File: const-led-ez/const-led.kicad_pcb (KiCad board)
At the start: 2 copper layers, 25.4 x 25.4 mm, 60 parts, among them CON1 AVR-ISP-6, J1 Micro_USB_B, J2 Conn_01x02, SW1 SW_SPST, SW2 SW_SPST, U1 MCP73831, U2 LM3410, U3 ATTINY85-20SU

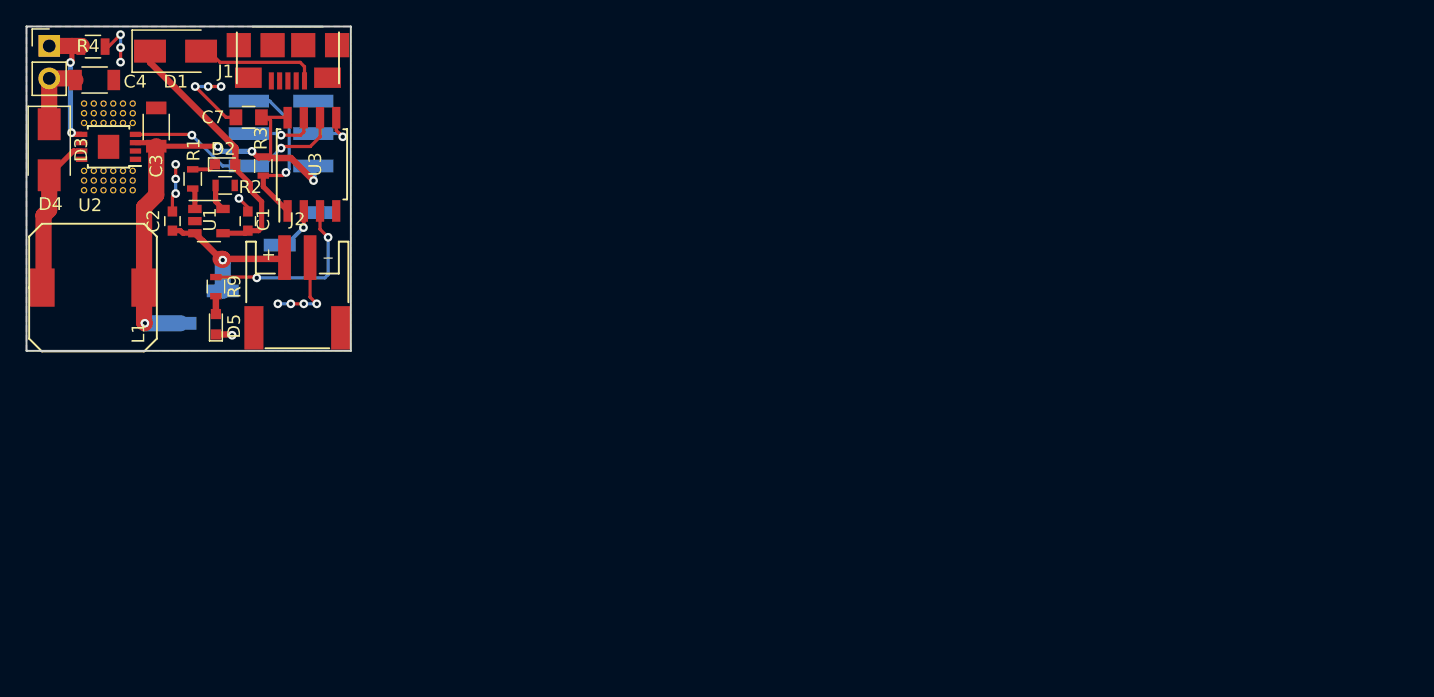
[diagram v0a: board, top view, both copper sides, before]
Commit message: Rev2
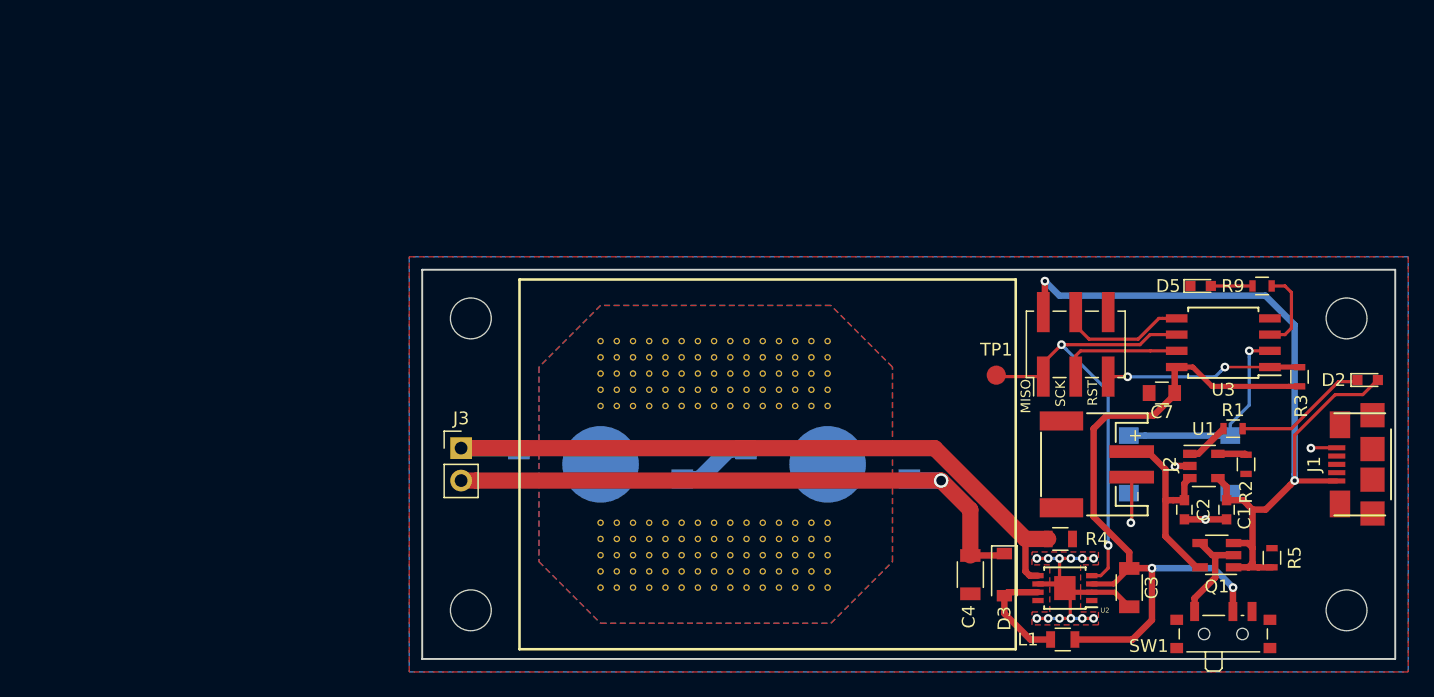
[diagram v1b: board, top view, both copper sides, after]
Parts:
- removed D1: D_Schottky, Diodes_SMD:D_SMA
- removed REF** (x36): VIA-12mil, personal_f:VIA-12mil
- added D6: LED, personal_f:ChanzonLED, B.Cu at (148.6, 111.8)
- added G***: LOGO, personal_f:Guang, B.Cu at (182.3, 111.8)
- added J3: Conn_01x02, Pin_Headers:Pin_Header_Straight_1x02_Pitch2.54mm, F.Cu at (137.7, 110.5)
- added J4: Conn_01x01, Mounting_Holes:MountingHole_3.2mm_M3, F.Cu at (138.4, 123.2)
- added J5: Conn_01x01, Mounting_Holes:MountingHole_3.2mm_M3, F.Cu at (207.0, 123.2)
- added J6: Conn_01x01, Mounting_Holes:MountingHole_3.2mm_M3, F.Cu at (138.4, 100.3)
- added J7: Conn_01x01, Mounting_Holes:MountingHole_3.2mm_M3, F.Cu at (207.0, 100.3)
- added J8: Conn_01x01, personal_f:VIA-12mil, F.Cu at (166.4, 121.4)
- added J8: Conn_01x01, personal_f:VIA-12mil, F.Cu at (154.9, 121.4)
- added J8: Conn_01x01, personal_f:VIA-12mil, F.Cu at (153.7, 121.4)
- added J8: Conn_01x01, personal_f:VIA-12mil, F.Cu at (152.4, 121.4)
- added J8: Conn_01x01, personal_f:VIA-12mil, F.Cu at (151.1, 121.4)
- added J8: Conn_01x01, personal_f:VIA-12mil, F.Cu at (149.9, 121.4)
- added J8: Conn_01x01, personal_f:VIA-12mil, F.Cu at (148.6, 121.4)
- added J8: Conn_01x01, personal_f:VIA-12mil, F.Cu at (166.4, 120.1)
- added J8: Conn_01x01, personal_f:VIA-12mil, F.Cu at (165.1, 120.1)
- added J8: Conn_01x01, personal_f:VIA-12mil, F.Cu at (163.8, 120.1)
- added J8: Conn_01x01, personal_f:VIA-12mil, F.Cu at (162.6, 120.1)
- added J8: Conn_01x01, personal_f:VIA-12mil, F.Cu at (165.1, 121.4)
- added J8: Conn_01x01, personal_f:VIA-12mil, F.Cu at (161.3, 120.1)
- added J8: Conn_01x01, personal_f:VIA-12mil, F.Cu at (160.0, 120.1)
- added J8: Conn_01x01, personal_f:VIA-12mil, F.Cu at (158.8, 120.1)
- added J8: Conn_01x01, personal_f:VIA-12mil, F.Cu at (157.5, 120.1)
- added J8: Conn_01x01, personal_f:VIA-12mil, F.Cu at (156.2, 120.1)
- added J8: Conn_01x01, personal_f:VIA-12mil, F.Cu at (154.9, 120.1)
- added J8: Conn_01x01, personal_f:VIA-12mil, F.Cu at (153.7, 120.1)
- added J8: Conn_01x01, personal_f:VIA-12mil, F.Cu at (152.4, 120.1)
- added J8: Conn_01x01, personal_f:VIA-12mil, F.Cu at (151.1, 120.1)
- added J8: Conn_01x01, personal_f:VIA-12mil, F.Cu at (149.9, 120.1)
- added J8: Conn_01x01, personal_f:VIA-12mil, F.Cu at (163.8, 121.4)
- added J8: Conn_01x01, personal_f:VIA-12mil, F.Cu at (148.6, 120.1)
- added J8: Conn_01x01, personal_f:VIA-12mil, F.Cu at (166.4, 118.9)
- added J8: Conn_01x01, personal_f:VIA-12mil, F.Cu at (165.1, 118.9)
- added J8: Conn_01x01, personal_f:VIA-12mil, F.Cu at (163.8, 118.9)
- added J8: Conn_01x01, personal_f:VIA-12mil, F.Cu at (162.6, 118.9)
- added J8: Conn_01x01, personal_f:VIA-12mil, F.Cu at (161.3, 118.9)
- added J8: Conn_01x01, personal_f:VIA-12mil, F.Cu at (160.0, 118.9)
- added J8: Conn_01x01, personal_f:VIA-12mil, F.Cu at (158.8, 118.9)
- added J8: Conn_01x01, personal_f:VIA-12mil, F.Cu at (157.5, 118.9)
- added J8: Conn_01x01, personal_f:VIA-12mil, F.Cu at (156.2, 118.9)
- added J8: Conn_01x01, personal_f:VIA-12mil, F.Cu at (162.6, 121.4)
- added J8: Conn_01x01, personal_f:VIA-12mil, F.Cu at (154.9, 118.9)
- added J8: Conn_01x01, personal_f:VIA-12mil, F.Cu at (153.7, 118.9)
- added J8: Conn_01x01, personal_f:VIA-12mil, F.Cu at (152.4, 118.9)
- added J8: Conn_01x01, personal_f:VIA-12mil, F.Cu at (151.1, 118.9)
- added J8: Conn_01x01, personal_f:VIA-12mil, F.Cu at (149.9, 118.9)
- added J8: Conn_01x01, personal_f:VIA-12mil, F.Cu at (148.6, 118.9)
- added J8: Conn_01x01, personal_f:VIA-12mil, F.Cu at (166.4, 117.6)
- added J8: Conn_01x01, personal_f:VIA-12mil, F.Cu at (165.1, 117.6)
- added J8: Conn_01x01, personal_f:VIA-12mil, F.Cu at (163.8, 117.6)
- added J8: Conn_01x01, personal_f:VIA-12mil, F.Cu at (162.6, 117.6)
- added J8: Conn_01x01, personal_f:VIA-12mil, F.Cu at (161.3, 121.4)
- added J8: Conn_01x01, personal_f:VIA-12mil, F.Cu at (161.3, 117.6)
- added J8: Conn_01x01, personal_f:VIA-12mil, F.Cu at (160.0, 117.6)
- added J8: Conn_01x01, personal_f:VIA-12mil, F.Cu at (158.8, 117.6)
- added J8: Conn_01x01, personal_f:VIA-12mil, F.Cu at (157.5, 117.6)
- added J8: Conn_01x01, personal_f:VIA-12mil, F.Cu at (156.2, 117.6)
- added J8: Conn_01x01, personal_f:VIA-12mil, F.Cu at (154.9, 117.6)
- added J8: Conn_01x01, personal_f:VIA-12mil, F.Cu at (153.7, 117.6)
- added J8: Conn_01x01, personal_f:VIA-12mil, F.Cu at (152.4, 117.6)
- added J8: Conn_01x01, personal_f:VIA-12mil, F.Cu at (151.1, 117.6)
- added J8: Conn_01x01, personal_f:VIA-12mil, F.Cu at (149.9, 117.6)
- added J8: Conn_01x01, personal_f:VIA-12mil, F.Cu at (160.0, 121.4)
- added J8: Conn_01x01, personal_f:VIA-12mil, F.Cu at (148.6, 117.6)
- added J8: Conn_01x01, personal_f:VIA-12mil, F.Cu at (166.4, 116.3)
- added J8: Conn_01x01, personal_f:VIA-12mil, F.Cu at (165.1, 116.3)
- added J8: Conn_01x01, personal_f:VIA-12mil, F.Cu at (163.8, 116.3)
- added J8: Conn_01x01, personal_f:VIA-12mil, F.Cu at (162.6, 116.3)
- added J8: Conn_01x01, personal_f:VIA-12mil, F.Cu at (161.3, 116.3)
- added J8: Conn_01x01, personal_f:VIA-12mil, F.Cu at (160.0, 116.3)
- added J8: Conn_01x01, personal_f:VIA-12mil, F.Cu at (158.8, 116.3)
- added J8: Conn_01x01, personal_f:VIA-12mil, F.Cu at (157.5, 116.3)
- added J8: Conn_01x01, personal_f:VIA-12mil, F.Cu at (156.2, 116.3)
- added J8: Conn_01x01, personal_f:VIA-12mil, F.Cu at (158.8, 121.4)
- added J8: Conn_01x01, personal_f:VIA-12mil, F.Cu at (154.9, 116.3)
- added J8: Conn_01x01, personal_f:VIA-12mil, F.Cu at (153.7, 116.3)
- added J8: Conn_01x01, personal_f:VIA-12mil, F.Cu at (152.4, 116.3)
- added J8: Conn_01x01, personal_f:VIA-12mil, F.Cu at (151.1, 116.3)
- added J8: Conn_01x01, personal_f:VIA-12mil, F.Cu at (149.9, 116.3)
- added J8: Conn_01x01, personal_f:VIA-12mil, F.Cu at (148.6, 116.3)
- added J8: Conn_01x01, personal_f:VIA-12mil, F.Cu at (157.5, 121.4)
- added J8: Conn_01x01, personal_f:VIA-12mil, F.Cu at (156.2, 121.4)
- added J9: Conn_01x01, personal_f:VIA-12mil, F.Cu at (166.4, 102.1)
- added J9: Conn_01x01, personal_f:VIA-12mil, F.Cu at (154.9, 102.1)
- added J9: Conn_01x01, personal_f:VIA-12mil, F.Cu at (153.7, 102.1)
- added J9: Conn_01x01, personal_f:VIA-12mil, F.Cu at (152.4, 102.1)
- added J9: Conn_01x01, personal_f:VIA-12mil, F.Cu at (151.1, 102.1)
- added J9: Conn_01x01, personal_f:VIA-12mil, F.Cu at (149.9, 102.1)
- added J9: Conn_01x01, personal_f:VIA-12mil, F.Cu at (148.6, 102.1)
- added J9: Conn_01x01, personal_f:VIA-12mil, F.Cu at (166.4, 103.4)
- added J9: Conn_01x01, personal_f:VIA-12mil, F.Cu at (165.1, 103.4)
- added J9: Conn_01x01, personal_f:VIA-12mil, F.Cu at (163.8, 103.4)
- added J9: Conn_01x01, personal_f:VIA-12mil, F.Cu at (162.6, 103.4)
- added J9: Conn_01x01, personal_f:VIA-12mil, F.Cu at (165.1, 102.1)
- added J9: Conn_01x01, personal_f:VIA-12mil, F.Cu at (161.3, 103.4)
- added J9: Conn_01x01, personal_f:VIA-12mil, F.Cu at (160.0, 103.4)
- added J9: Conn_01x01, personal_f:VIA-12mil, F.Cu at (158.8, 103.4)
- added J9: Conn_01x01, personal_f:VIA-12mil, F.Cu at (157.5, 103.4)
- added J9: Conn_01x01, personal_f:VIA-12mil, F.Cu at (156.2, 103.4)
- added J9: Conn_01x01, personal_f:VIA-12mil, F.Cu at (154.9, 103.4)
- added J9: Conn_01x01, personal_f:VIA-12mil, F.Cu at (153.7, 103.4)
- added J9: Conn_01x01, personal_f:VIA-12mil, F.Cu at (152.4, 103.4)
- added J9: Conn_01x01, personal_f:VIA-12mil, F.Cu at (151.1, 103.4)
- added J9: Conn_01x01, personal_f:VIA-12mil, F.Cu at (149.9, 103.4)
- added J9: Conn_01x01, personal_f:VIA-12mil, F.Cu at (163.8, 102.1)
- added J9: Conn_01x01, personal_f:VIA-12mil, F.Cu at (148.6, 103.4)
- added J9: Conn_01x01, personal_f:VIA-12mil, F.Cu at (166.4, 104.6)
- added J9: Conn_01x01, personal_f:VIA-12mil, F.Cu at (165.1, 104.6)
- added J9: Conn_01x01, personal_f:VIA-12mil, F.Cu at (163.8, 104.6)
- added J9: Conn_01x01, personal_f:VIA-12mil, F.Cu at (162.6, 104.6)
- added J9: Conn_01x01, personal_f:VIA-12mil, F.Cu at (161.3, 104.6)
- added J9: Conn_01x01, personal_f:VIA-12mil, F.Cu at (160.0, 104.6)
- added J9: Conn_01x01, personal_f:VIA-12mil, F.Cu at (158.8, 104.6)
- added J9: Conn_01x01, personal_f:VIA-12mil, F.Cu at (157.5, 104.6)
- added J9: Conn_01x01, personal_f:VIA-12mil, F.Cu at (156.2, 104.6)
- added J9: Conn_01x01, personal_f:VIA-12mil, F.Cu at (162.6, 102.1)
- added J9: Conn_01x01, personal_f:VIA-12mil, F.Cu at (154.9, 104.6)
- added J9: Conn_01x01, personal_f:VIA-12mil, F.Cu at (153.7, 104.6)
- added J9: Conn_01x01, personal_f:VIA-12mil, F.Cu at (152.4, 104.6)
- added J9: Conn_01x01, personal_f:VIA-12mil, F.Cu at (151.1, 104.6)
- added J9: Conn_01x01, personal_f:VIA-12mil, F.Cu at (149.9, 104.6)
- added J9: Conn_01x01, personal_f:VIA-12mil, F.Cu at (148.6, 104.6)
- added J9: Conn_01x01, personal_f:VIA-12mil, F.Cu at (166.4, 105.9)
- added J9: Conn_01x01, personal_f:VIA-12mil, F.Cu at (165.1, 105.9)
- added J9: Conn_01x01, personal_f:VIA-12mil, F.Cu at (163.8, 105.9)
- added J9: Conn_01x01, personal_f:VIA-12mil, F.Cu at (162.6, 105.9)
- added J9: Conn_01x01, personal_f:VIA-12mil, F.Cu at (161.3, 102.1)
- added J9: Conn_01x01, personal_f:VIA-12mil, F.Cu at (161.3, 105.9)
- added J9: Conn_01x01, personal_f:VIA-12mil, F.Cu at (160.0, 105.9)
- added J9: Conn_01x01, personal_f:VIA-12mil, F.Cu at (158.8, 105.9)
- added J9: Conn_01x01, personal_f:VIA-12mil, F.Cu at (157.5, 105.9)
- added J9: Conn_01x01, personal_f:VIA-12mil, F.Cu at (156.2, 105.9)
- added J9: Conn_01x01, personal_f:VIA-12mil, F.Cu at (154.9, 105.9)
- added J9: Conn_01x01, personal_f:VIA-12mil, F.Cu at (153.7, 105.9)
- added J9: Conn_01x01, personal_f:VIA-12mil, F.Cu at (152.4, 105.9)
- added J9: Conn_01x01, personal_f:VIA-12mil, F.Cu at (151.1, 105.9)
- added J9: Conn_01x01, personal_f:VIA-12mil, F.Cu at (149.9, 105.9)
- added J9: Conn_01x01, personal_f:VIA-12mil, F.Cu at (160.0, 102.1)
- added J9: Conn_01x01, personal_f:VIA-12mil, F.Cu at (148.6, 105.9)
- added J9: Conn_01x01, personal_f:VIA-12mil, F.Cu at (166.4, 107.2)
- added J9: Conn_01x01, personal_f:VIA-12mil, F.Cu at (165.1, 107.2)
- added J9: Conn_01x01, personal_f:VIA-12mil, F.Cu at (163.8, 107.2)
- added J9: Conn_01x01, personal_f:VIA-12mil, F.Cu at (162.6, 107.2)
- added J9: Conn_01x01, personal_f:VIA-12mil, F.Cu at (161.3, 107.2)
- added J9: Conn_01x01, personal_f:VIA-12mil, F.Cu at (160.0, 107.2)
- added J9: Conn_01x01, personal_f:VIA-12mil, F.Cu at (158.8, 107.2)
- added J9: Conn_01x01, personal_f:VIA-12mil, F.Cu at (157.5, 107.2)
- added J9: Conn_01x01, personal_f:VIA-12mil, F.Cu at (156.2, 107.2)
- added J9: Conn_01x01, personal_f:VIA-12mil, F.Cu at (158.8, 102.1)
- added J9: Conn_01x01, personal_f:VIA-12mil, F.Cu at (154.9, 107.2)
- added J9: Conn_01x01, personal_f:VIA-12mil, F.Cu at (153.7, 107.2)
- added J9: Conn_01x01, personal_f:VIA-12mil, F.Cu at (152.4, 107.2)
- added J9: Conn_01x01, personal_f:VIA-12mil, F.Cu at (151.1, 107.2)
- added J9: Conn_01x01, personal_f:VIA-12mil, F.Cu at (149.9, 107.2)
- added J9: Conn_01x01, personal_f:VIA-12mil, F.Cu at (148.6, 107.2)
- added J9: Conn_01x01, personal_f:VIA-12mil, F.Cu at (157.5, 102.1)
- added J9: Conn_01x01, personal_f:VIA-12mil, F.Cu at (156.2, 102.1)
- added Q1: QS5U28, TO_SOT_Packages_SMD:TSOT-23-5, F.Cu at (196.8, 118.9)
- added R5: 100k, Resistors_SMD:R_0603, F.Cu at (201.2, 119.1)
- added TP1: TEST, Measurement_Points:Measurement_Point_Round-SMD-Pad_Small, F.Cu at (179.6, 104.8)
- CON1: moved to F.Cu
- D3: value D_Schottky -> 1N5819; footprint Diodes_SMD:D_SMA -> Diodes_SMD:D_SOD-123
- D4: footprint Pin_Headers:Pin_Header_Straight_1x02_Pitch2.54mm -> personal_f:ChanzonLED; moved to B.Cu
- L1: value 16u -> 4u; footprint personal_f:muRata_L -> Inductors_SMD:L_0805
- R9: value R -> 1k
- SW1: footprint Pin_Headers:Pin_Header_Straight_1x02_Pitch2.54mm_SMD_Pin1Left -> Buttons_Switches_SMD:SW_SPDT_PCM12; moved to F.Cu
- SW2: footprint Pin_Headers:Pin_Header_Straight_1x02_Pitch2.54mm_SMD_Pin1Left -> Buttons_Switches_SMD:SW_SPST_B3S-1000
- moved J1 91.1 mm to (209.0, 111.8), turned to 90 degrees
- moved D2 91.1 mm to (208.7, 105.2)
- moved R4 85.0 mm to (184.6, 117.6)
- moved C3 84.3 mm to (190.0, 121.4), turned to 270 degrees
- moved SW1 83.9 mm to (197.4, 124.7), turned to 0 degrees
- moved R1 83.8 mm to (198.1, 109.0), turned to 0 degrees
- moved R2 82.9 mm to (199.1, 111.8), turned to 270 degrees
- moved R3 82.8 mm to (203.3, 104.9), turned to 90 degrees
- moved U2 82.5 mm to (185.0, 121.5)
- moved C2 82.4 mm to (194.3, 115.3), turned to 270 degrees
- moved R9 81.9 mm to (200.4, 97.8), turned to 180 degrees
- moved D3 81.9 mm to (180.2, 120.4)
- moved L1 80.8 mm to (184.8, 125.5), turned to 180 degrees
- moved U1 80.2 mm to (195.8, 111.9)
- moved C1 79.9 mm to (197.6, 115.3), turned to 270 degrees
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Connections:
- C1 pad 1: /VIN -> V_USB
- CON1 pad 2: VCC -> V_USB
- D2 pad 2: /VIN -> V_USB
- D4 pad 1: /FB -> Net-(D4-Pad1)
- J1 pad 1: Net-(D1-Pad2) -> V_USB
- J1 pad 2: Net-(J1-Pad2) -> (no net)
- J1 pad 3: Net-(J1-Pad3) -> (no net)
- J1 pad 4: Net-(J1-Pad4) -> (no net)
- SW1 pad 1: /VBAT -> Net-(Q1-Pad2)
- U1 pad 4: /VIN -> V_USB
- U2 pad 1: Net-(U2-Pad1) -> (no net)
- U2 pad 8: Net-(U2-Pad8) -> (no net)
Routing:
- net V_USB: track 0.00 -> 68.6 mm, vias 0 -> 2
- net /FB: track 10.3 -> 57.2 mm, vias 2 -> 0
- net Net-(C4-Pad1): track 5.70 -> 49.7 mm, vias 0 -> 1
- net /VIN: track 20.6 -> 0.00 mm
- net /MISO: track 18.4 -> 36.8 mm
- net VCC: track 40.7 -> 56.8 mm, vias 4 -> 2
- net Net-(SW2-Pad2): track 3.73 -> 16.8 mm
- net Net-(D1-Pad2): track 9.71 -> 0.00 mm
- net Net-(D2-Pad1): track 1.90 -> 10.4 mm
- net Net-(Q1-Pad2): track 0.00 -> 8.09 mm
- net Net-(R9-Pad1): track 14.2 -> 6.45 mm, vias 2 -> 0
- net GND: track 23.4 -> 29.7 mm, vias 15 -> 16
- net /MOSI: track 4.11 -> 10.1 mm, vias 1 -> 0
- net Net-(D4-Pad1): track 0.00 -> 5.93 mm
- net /SCK: track 5.57 -> 9.70 mm, vias 1 -> 0
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- added copper zone on B.Cu, net /THERM
- added copper zone on F.Cu, net /THERM
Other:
- board size 25.4 x 25.4 mm -> 76.2 x 30.5 mm
- rule via_min_drill: 0.3302 -> 0.254
- rule via_min_size: 0.6858 -> 0.4572
- board text added: "Jeffrey Ni PortaLED v2 2018"
- board text removed: "LED Driver J. Ni 2018"
- board text removed: "VCC"
